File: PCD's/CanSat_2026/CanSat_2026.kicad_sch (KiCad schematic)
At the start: 9 parts, among them J1 Conn_01x02_Pin, J2 Conn_01x06, J3 Conn_01x06, J4 9DOF, J5 Conn_01x03_Pin, U1 LM1085-3.3, U2 LP5907MFX-1.8, U3 ESP32-WROOM-32D, U4 SN74AVC4T245PW

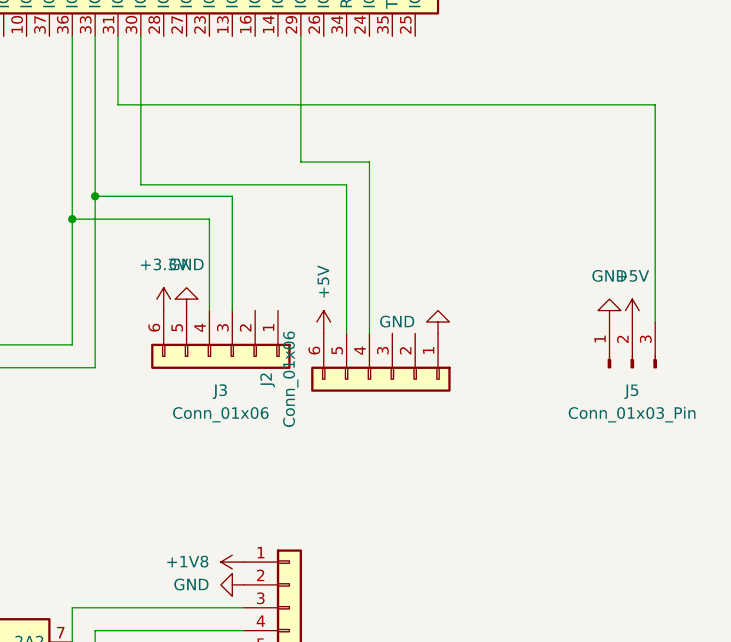
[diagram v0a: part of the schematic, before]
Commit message: update to pcb
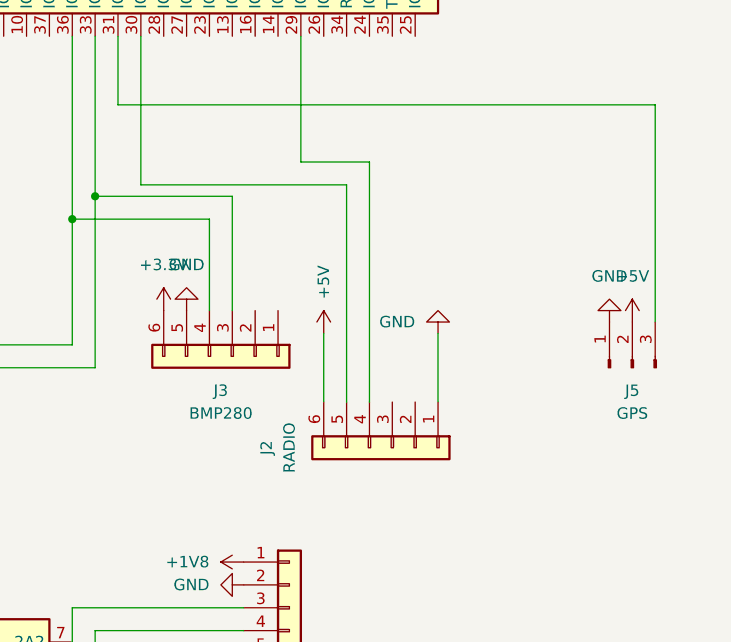
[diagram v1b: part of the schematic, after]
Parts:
- J2: value Conn_01x06 -> RADIO
- J3: value Conn_01x06 -> BMP280
- J5: value Conn_01x03_Pin -> GPS
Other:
- moved on the sheet: J2
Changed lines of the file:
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@@
 	(wire
 		(pts
-			(xy 172.72 123.19) (xy 172.72 106.68)
-		)
-		(stroke
-			(width 0)
-			(type default)
-		)
-	)
-	(wire
-		(pts
-			(xy 175.26 123.19) (xy 175.26 104.14)
+			(xy 172.72 130.81) (xy 172.72 106.68)
+		)
+		(stroke
+			(width 0)
+			(type default)
+		)
+	)
+	(wire
+		(pts
+			(xy 175.26 130.81) (xy 175.26 104.14)
 		)
 		(stroke
@@
 	(wire
 		(pts
+			(xy 170.18 130.81) (xy 170.18 123.19)
+		)
+		(stroke
+			(width 0)
+			(type default)
+		)
+	)
+	(wire
+		(pts
 			(xy 160.02 107.95) (xy 144.78 107.95)
 		)
@@
 		(pts
 			(xy 172.72 106.68) (xy 149.86 106.68)
+		)
+		(stroke
+			(width 0)
+			(type default)
+		)
+	)
+	(wire
+		(pts
+			(xy 182.88 130.81) (xy 182.88 123.19)
 		)
 		(stroke
@@
 			)
 		)
-		(property "Value" "Conn_01x03_Pin"
+		(property "Value" "GPS"
 			(at 204.47 132.08 90)
 			(effects
@@
 			)
 		)
-		(property "Value" "Conn_01x06"
+		(property "Value" "BMP280"
 			(at 158.75 132.08 90)
 			(effects
@@
 	(symbol
 		(lib_id "Connector_Generic:Conn_01x06")
-		(at 177.8 128.27 270)
+		(at 177.8 135.89 270)
 		(unit 1)
 		(exclude_from_sim no)
@@
 		(dnp no)
 		(property "Reference" "J2"
-			(at 163.83 128.27 0)
-			(effects
-				(font
-					(size 1.27 1.27)
-				)
-			)
-		)
-		(property "Value" "Conn_01x06"
-			(at 166.37 128.27 0)
+			(at 163.83 135.89 0)
+			(effects
+				(font
+					(size 1.27 1.27)
+				)
+			)
+		)
+		(property "Value" "RADIO"
+			(at 166.37 135.89 0)
 			(effects
 				(font
@@
 		)
 		(property "Footprint" "Connector_JST:JST_GH_SM06B-GHS-TB_1x06-1MP_P1.25mm_Horizontal"
-			(at 177.8 128.27 0)
+			(at 177.8 135.89 0)
 			(effects
 				(font
@@
 		)
 		(property "Datasheet" "~"
-			(at 177.8 128.27 0)
+			(at 177.8 135.89 0)
 			(effects
 				(font
@@
 		)
 		(property "Description" "Generic connector, single row, 01x06, script generated (kicad-library-utils/schlib/autogen/connector/)"
-			(at 177.8 128.27 0)
-			(effects
-				(font
+			(at 177.8 135.89 0)
+			(effects
+				(font
